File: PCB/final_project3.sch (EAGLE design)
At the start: 19 parts

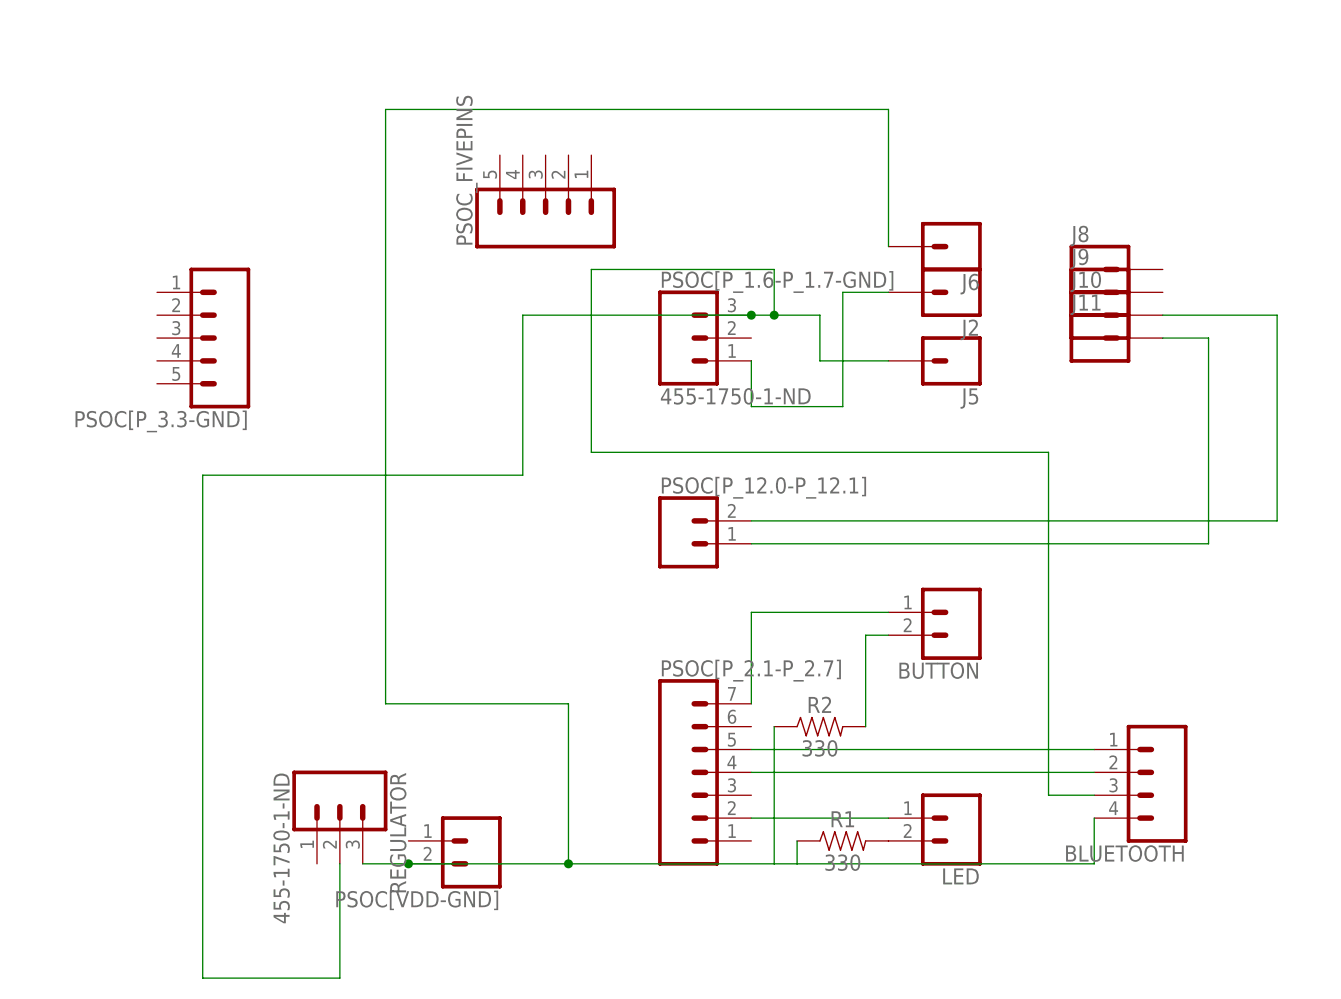
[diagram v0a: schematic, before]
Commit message: Final
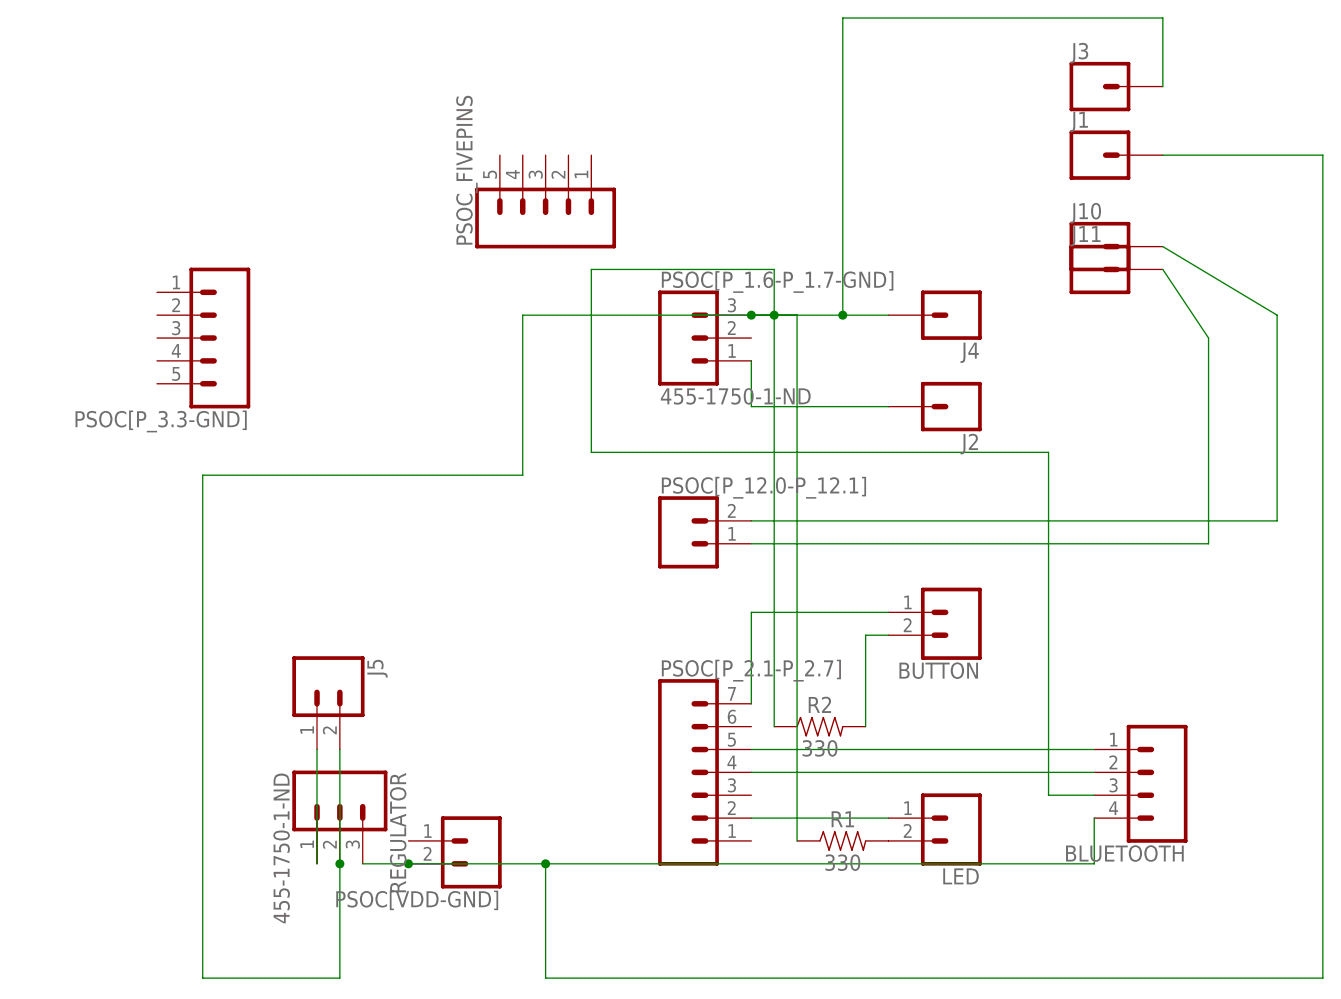
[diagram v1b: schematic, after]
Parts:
- removed J6, J8, J9: (no value), SparkFun-Connectors:CONN_01
- added J1, J3, J4: (no value), SparkFun-Connectors:CONN_01
- J5: device SparkFun-Connectors:CONN_01 -> SparkFun-Connectors:CONN_02
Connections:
- new net N$1: J5.1, REGULATOR.1
- net GND3: now also J3.1, J4.1, J5.2, R1.1, R2.1; no longer J5.1
- net VDD: now also J1.1; no longer J6.1, R1.1, R2.1
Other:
- moved on the sheet: J10, J11, J2
